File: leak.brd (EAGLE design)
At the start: 50 x 50 mm, 44 parts, among them IC1 74HC595D, IC2 74HC595D, IC3 ADA4692-2R, IC4 ADA4692-2R, U1 TPS72301DBVRSOT-23-5, U2 TLV703

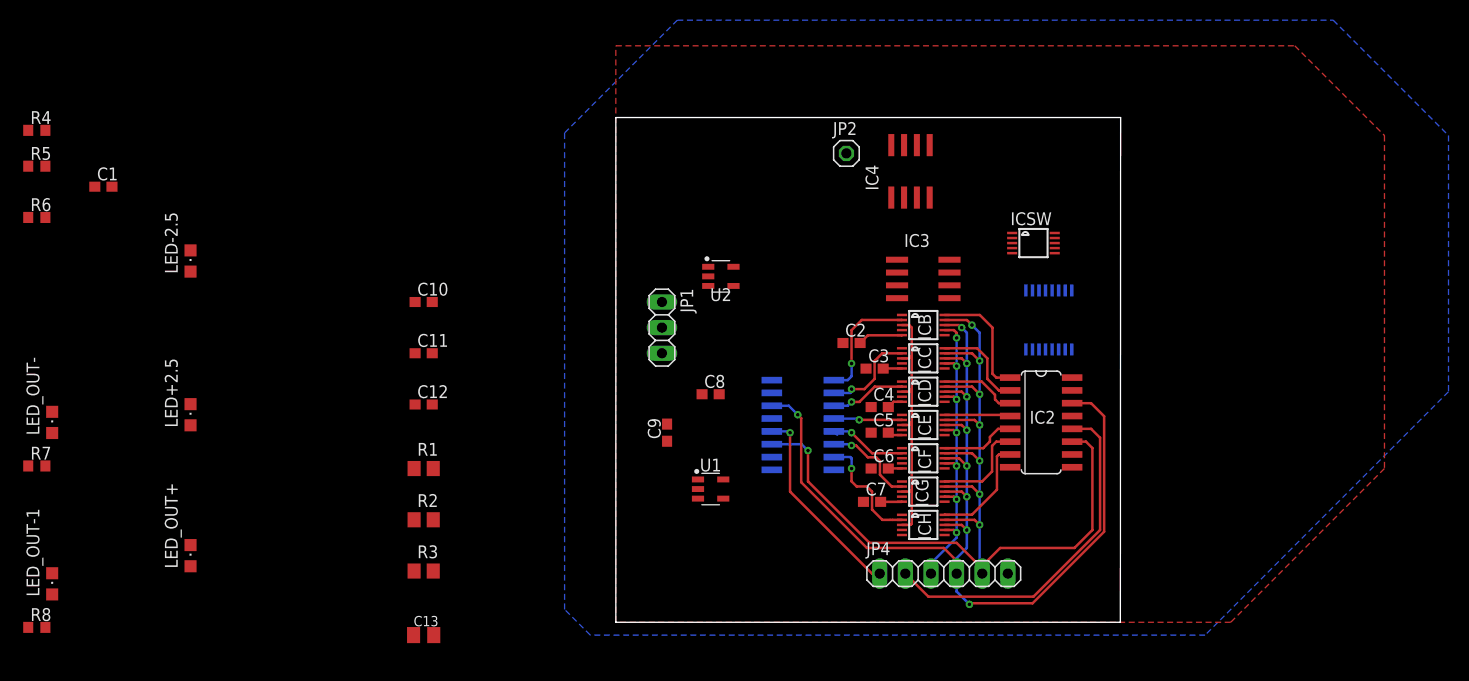
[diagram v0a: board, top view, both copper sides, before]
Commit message: v1 finished
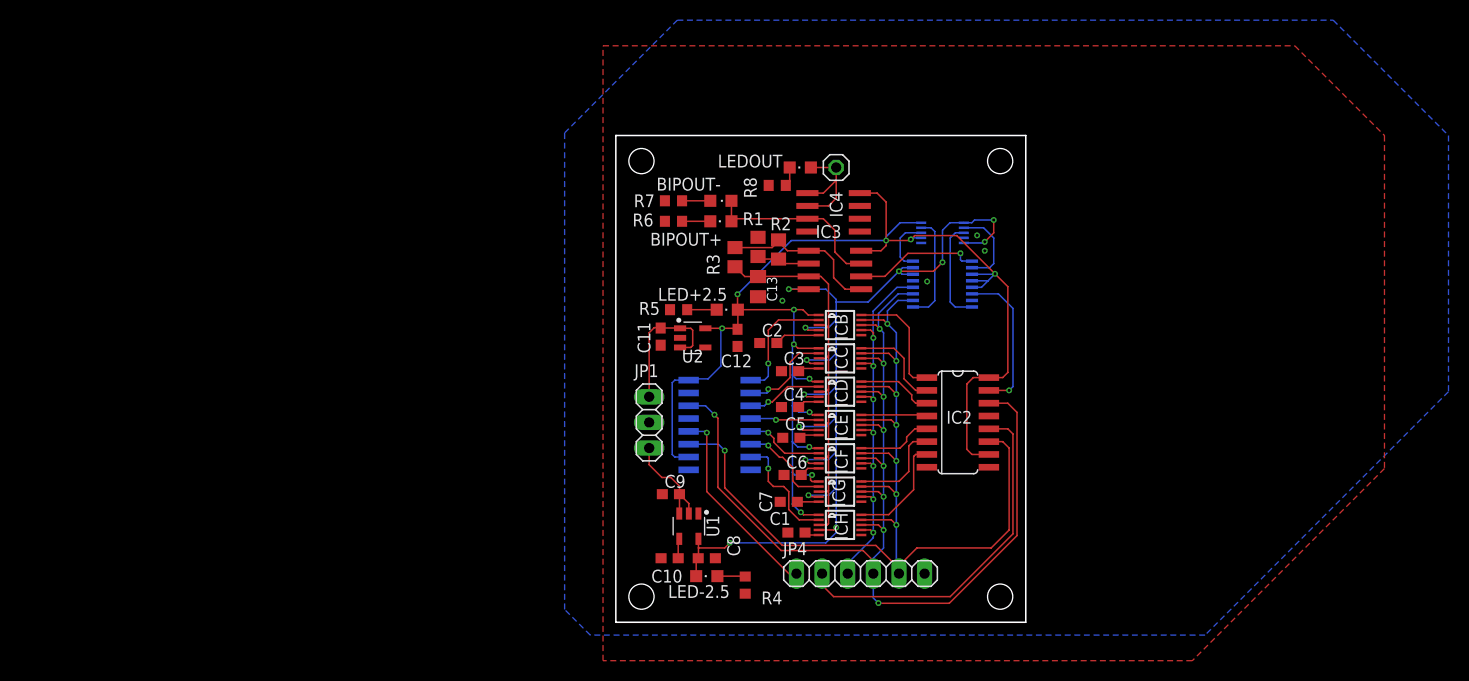
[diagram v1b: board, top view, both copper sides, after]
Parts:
- removed LED_OUT+, LED_OUT-, LED_OUT-1: (no value), led:CHIPLED_0805
- added BIPOUT+, BIPOUT-, LEDOUT: (no value), led:CHIPLED_0805
- moved R8 85.5 mm to (16.0, 43.3)
- moved R4 83.5 mm to (12.8, 3.68), turned to 90 degrees
- moved C1 76.8 mm to (17.9, 8.89)
- moved R7 68.4 mm to (5.71, 41.8)
- moved R5 65.2 mm to (6.22, 31.0)
- moved R6 63.1 mm to (5.71, 39.8)
- moved LED-2.5 60.0 mm to (9.02, 4.57), turned to 90 degrees
- moved LED+2.5 54.2 mm to (11.0, 31.0), turned to 90 degrees
- moved C13 47.9 mm to (14.1, 33.3), turned to 270 degrees
- moved R2 44.2 mm to (16.1, 37.0), turned to 90 degrees
- moved R3 43.8 mm to (11.8, 36.2), turned to 90 degrees
- moved R1 39.8 mm to (14.1, 37.2), turned to 270 degrees
- moved C10 35.2 mm to (5.33, 6.35)
- moved C12 31.8 mm to (12.1, 28.2), turned to 90 degrees
- moved C11 23.6 mm to (4.45, 28.3), turned to 90 degrees
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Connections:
- removed net AQA: IC1.15
- new net OUT_BIP: BIPOUT+.A, BIPOUT-.C, IC3.7, IC4.3
- net +2V5: now also ICSW.10
- net +5V: no longer ICSW.10
- net -2V5: now also ICSW.5
- net -5V: no longer ICSW.5
- net N$10: now also BIPOUT-.A; no longer LED_OUT-.A
- net N$12: now also LEDOUT.C; no longer LED_OUT-1.C
- net N$9: now also BIPOUT+.C; no longer LED_OUT+.C
- net OUT: now also LEDOUT.A; no longer IC3.7, IC4.3, LED_OUT+.A, LED_OUT-.C, LED_OUT-1.A
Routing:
- net +2V5: track 0.00 -> 145.7 mm, vias 0 -> 12
- net -2V5: track 0.00 -> 108.1 mm, vias 0 -> 13
- net OUT_BIP: track 0.00 -> 18.1 mm
- net N$2: track 0.00 -> 16.0 mm
- net W: track 25.8 -> 41.2 mm
- net CSA: track 0.00 -> 14.9 mm, vias 0 -> 1
- net +5V: track 0.00 -> 13.8 mm
- net LVLW: track 0.00 -> 12.6 mm, vias 0 -> 1
- net OUT: track 0.00 -> 12.1 mm
- net O1: track 0.00 -> 10.8 mm
- net -5V: track 0.00 -> 10.6 mm
- net O2: track 0.00 -> 10.3 mm
- net LVLA: track 0.00 -> 8.25 mm
- net MISO: track 34.0 -> 41.6 mm
- net MOSI: track 106.2 -> 112.2 mm
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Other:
- board size 50 x 50 mm -> 40.6 x 48.3 mm
